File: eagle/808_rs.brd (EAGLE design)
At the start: 100 x 80 mm, 75 parts, among them IC1 TL072P, IC2 TL072P, Q1 2SK30, Q59 2N3904, Q60 2N3906, Q61 2N3904, Q62 2N3904, Q63 2N3904, SW8 808_LT_MSS42_SW_4PDT

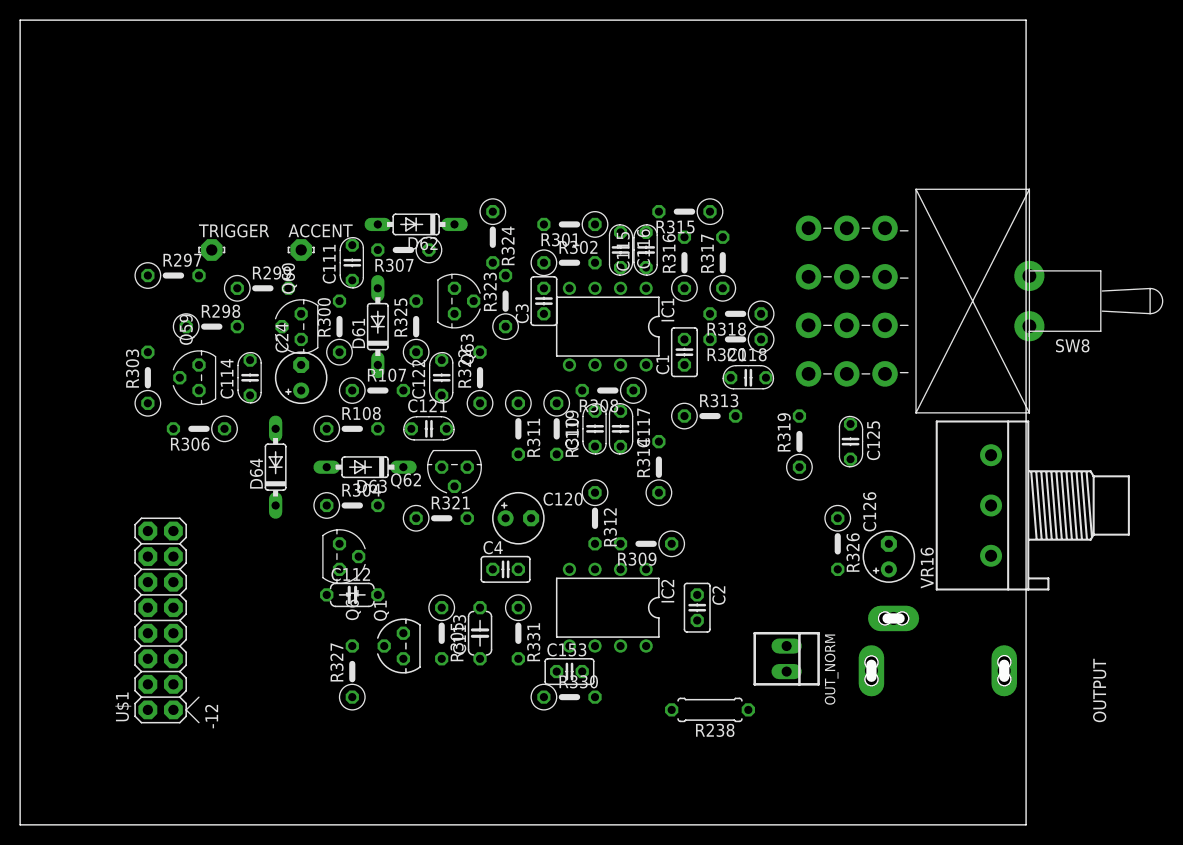
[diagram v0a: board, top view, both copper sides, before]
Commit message: working up to route
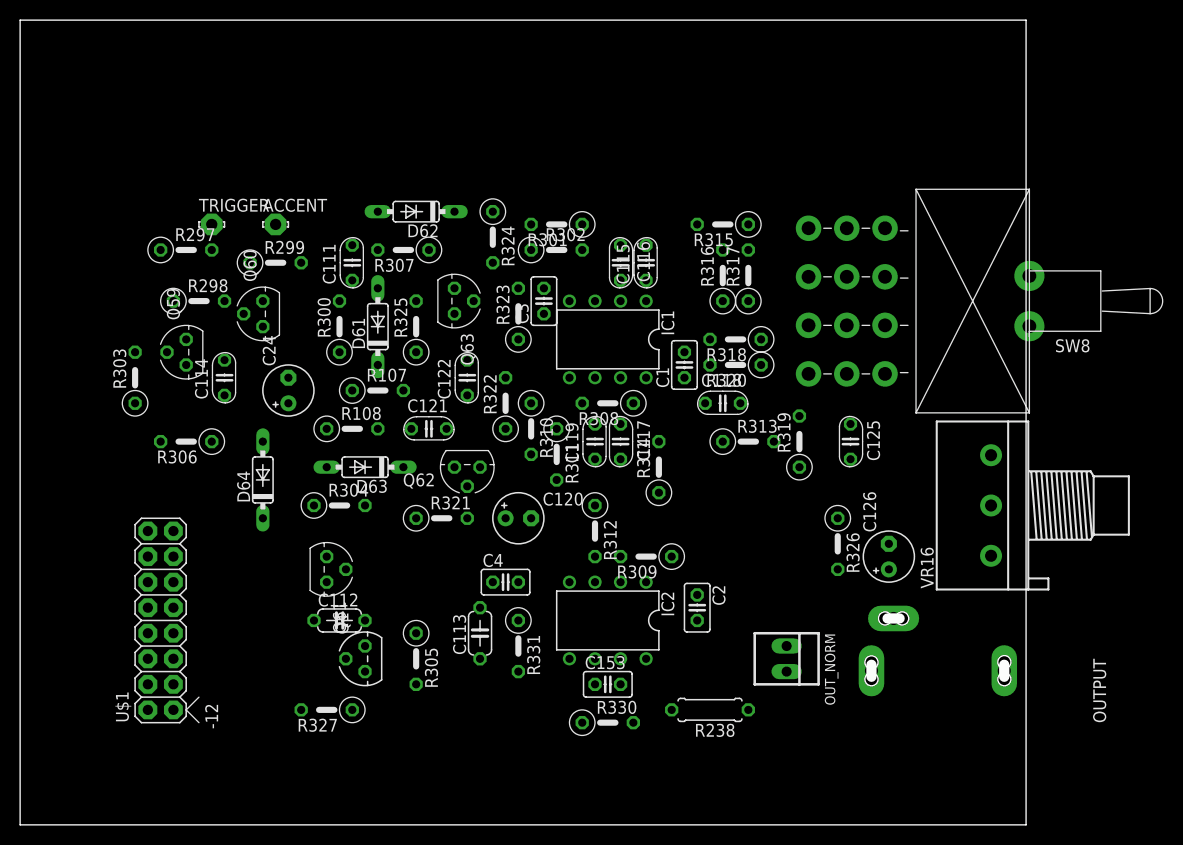
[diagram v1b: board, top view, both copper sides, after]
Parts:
- moved R311 4.58 mm to (53.3, 36.8)
- moved R313 4.58 mm to (72.4, 38.1)
- moved R327 4.58 mm to (30.5, 11.4), turned to 180 degrees
- moved R330 4.58 mm to (58.4, 10.2)
- moved C153 4.02 mm to (58.4, 14.0)
- moved Q1 4.02 mm to (34.3, 16.5)
- moved Q60 4.02 mm to (24.1, 50.8)
- moved R315 4.02 mm to (69.8, 59.7)
- moved R316 4.02 mm to (69.8, 54.6)
- moved C118 3.59 mm to (69.8, 41.9)
- moved R322 3.59 mm to (48.3, 41.9)
- moved ACCENT 3.59 mm to (25.4, 59.7)
- moved R305 3.59 mm to (39.4, 16.5)
- moved R317 2.84 mm to (72.4, 54.6)
- moved C112 2.84 mm to (31.8, 20.3)
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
